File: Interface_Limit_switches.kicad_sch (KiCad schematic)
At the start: 0 parts

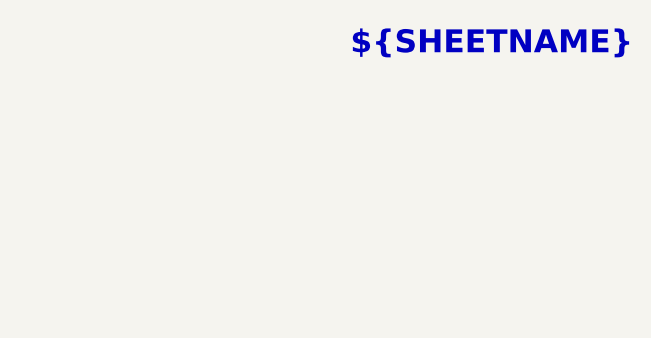
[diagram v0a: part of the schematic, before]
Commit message: testing green mask
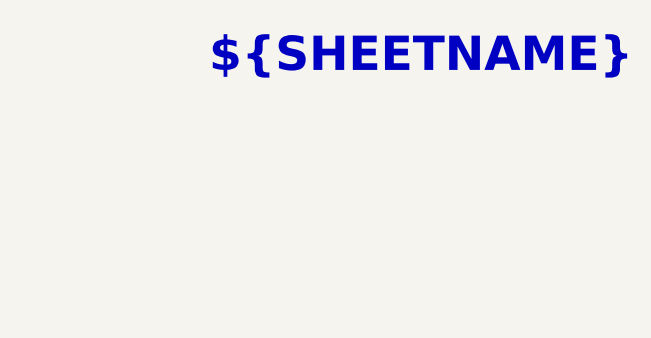
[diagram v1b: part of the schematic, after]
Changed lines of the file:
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@@
 	(generator_version "10.0")
 	(paper "A4")
-	(text "${SHEETNAME}"
-		(exclude_from_sim no)
-		(at 283.21 13.97 0)
-		(effects
-			(font
-				(size 2.54 2.54)
-				(bold yes)
-			)
-			(justify right top)
-		)
-	)
 	(text "JST B4B XH A / JST XHP-4 connector\n\nPin  Description\n  1  Bottom limit switch (Normally open, switch closes to GND)\n  2  GND\n  3  GND\n  4  Top limit switch (Normally open, switch closes to GND)"
 		(exclude_from_sim no)
@@
 		)
 	)
+	(text "${SHEETNAME}"
+		(exclude_from_sim no)
+		(at 283.21 14.605 0)
+		(effects
+			(font
+				(face "DejaVu Sans")
+				(size 3.81 3.81)
+				(bold yes)
+				(color 0 0 0 1)
+			)
+			(justify right top)
+		)
+	)
